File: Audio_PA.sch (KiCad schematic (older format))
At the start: 0 parts

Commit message: Electric circuit Ver_1
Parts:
- added C? (x2): 1uF, symbol C
- added C?: 330pF, symbol C
- added C?: 47uF, symbol CP1
- added C?: 10nF, symbol C
- added C? (x3): 100nF, symbol C
- added C?: 100uF, symbol CP1
- added C? (x2): 18pF, symbol C
- added C? (x2): 1000uF, symbol CP1
- added D? (x2): 15V, symbol D_Zener
- added D? (x2): 1N4148, symbol D
- added F? (x2): 3A, symbol Fuse
- added P?: Audio_In, symbol CONN_01X02
- added P?: -45VDC, symbol CONN_01X01
- added P?: Audio_Out, symbol CONN_01X02
- added P?: +45VDC, symbol CONN_01X01
- added Q? (x4): BCM856DS, symbol BCM856DS
- added Q? (x3): MJE350, symbol MJE350
- added Q? (x3): MJE340, symbol MJE340
- added Q?: BD139, symbol BD139
- added Q?: 2N3904, symbol Q_NPN_EBC
- added Q?: 2N3906, symbol Q_PNP_EBC
- added Q?: Q_NMOS_GDS, symbol Q_NMOS_GDS
- added Q?: Q_PMOS_GDS, symbol Q_PMOS_GDS
- added R?: 47K, symbol R
- added R?: 2K2, symbol R
- added R? (x3): 1K, symbol R
- added R? (x3): 470R, symbol R
- added R? (x4): 10K, symbol R
- added R? (x3): 100R, symbol R
- added R?: 27K, symbol R
- added R? (x2): 3K9, symbol R
- added R?: 10R, symbol R
- added R? (x4): R, symbol R
- added R? (x2): 0R33, symbol R
- added R? (x2): 330R, symbol R
- added RV?: 100R, symbol POT_TRIM
- added RV?: 1K, symbol POT_TRIM
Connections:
- new net: C?.1, C?.1, P?.1 (P1)
- new net: C?.2, C?.2, R?.1, R?.2
- new net: C?.1, Q?.2 (B), R?.1
- new net: Q?.1 (E), RV?.1
- new net: C?.2, Q?.3 (B), Q?.6 (C), R?.1
- new net: C?.1, Q?.3 (B), Q?.3 (C), R?.1
- new net: Q?.4 (E), RV?.3
- new net: Q?.5 (B), R?.1, R?.2
- new net: Q?.3 (C), RV?.2
- new net: C?.1, Q?.1 (E), Q?.1 (E), R?.1, R?.1, R?.1
- new net: Q?.2 (B), R?.1
- new net: Q?.5 (B), Q?.6 (C), R?.1
- new net: Q?.4 (E), R?.2, R?.2
- new net: C?.2, R?.1, R?.2
- new net: Q?.1 (E), R?.2 (x2)
- new net: Q?.2 (C), Q?.3 (B), Q?.3 (B), R?.1
- new net: C?.1, D?.1 (K), Q?.2 (C), Q?.2 (C), R?.1, R?.1
- new net: Q?.1 (E), Q?.1 (E), R?.1
- new net: C?.2, Q?.2 (C), R?.2
- new net: C?.1, C?.2, D?.2 (A), Q?.1 (E), Q?.2 (C), R?.1, R?.2
- new net: C?.1, C?.1, C?.1, R?.2
- new net: C?.1, D?.1 (K), D?.2 (A), P?.1 (P1), Q?.1 (E), Q?.1 (E), R?.1, R?.1, R?.1, R?.2, R?.2
- new net: Q?.1 (E), R?.2, R?.2, R?.2
- new net: F?.1, P?.1 (P1) (x2)
- new net: F?.2, Q?.2 (C), Q?.3 (S), R?.1
- new net: C?.2, R?.1
- new net: Q?.3 (B), R?.2, RV?.3
- new net: R?.1, RV?.1, RV?.2
- new net: D?.2 (A), Q?.1 (G), R?.2
- new net: D?.1 (K), Q?.1 (G), R?.2
- new net: D?.1 (K), Q?.3 (C)
- new net: D?.2 (A), Q?.3 (C)
- new net: Q?.2 (B), R?.1, R?.2 (x2)
- new net: Q?.3 (S), R?.1, R?.1
- new net: Q?.2 (D), R?.2, R?.2
- new net: F?.2, Q?.2 (C), Q?.2 (D), R?.1
- new net: C?.1, Q?.3 (B), R?.2
- new net: C?.2, Q?.3 (B), R?.2
- new net Earth: C?.1, C?.2, C?.2, C?.2, C?.2, P?.2 (P2), P?.2 (P2), R?.2, R?.2, R?.2

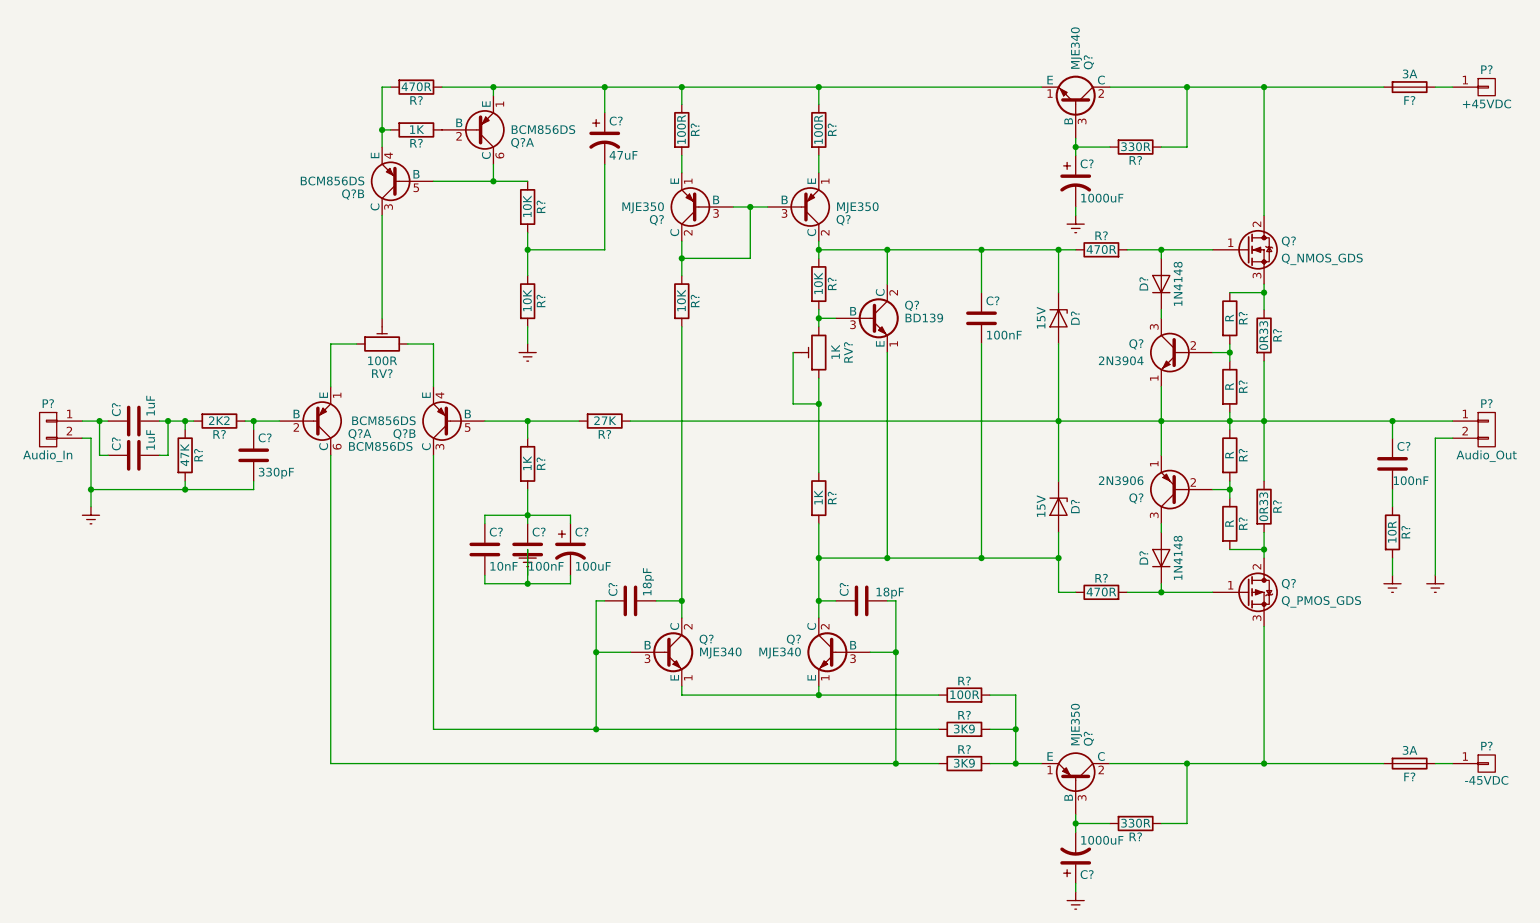
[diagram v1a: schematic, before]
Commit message: Electric circuit Ver_1.1
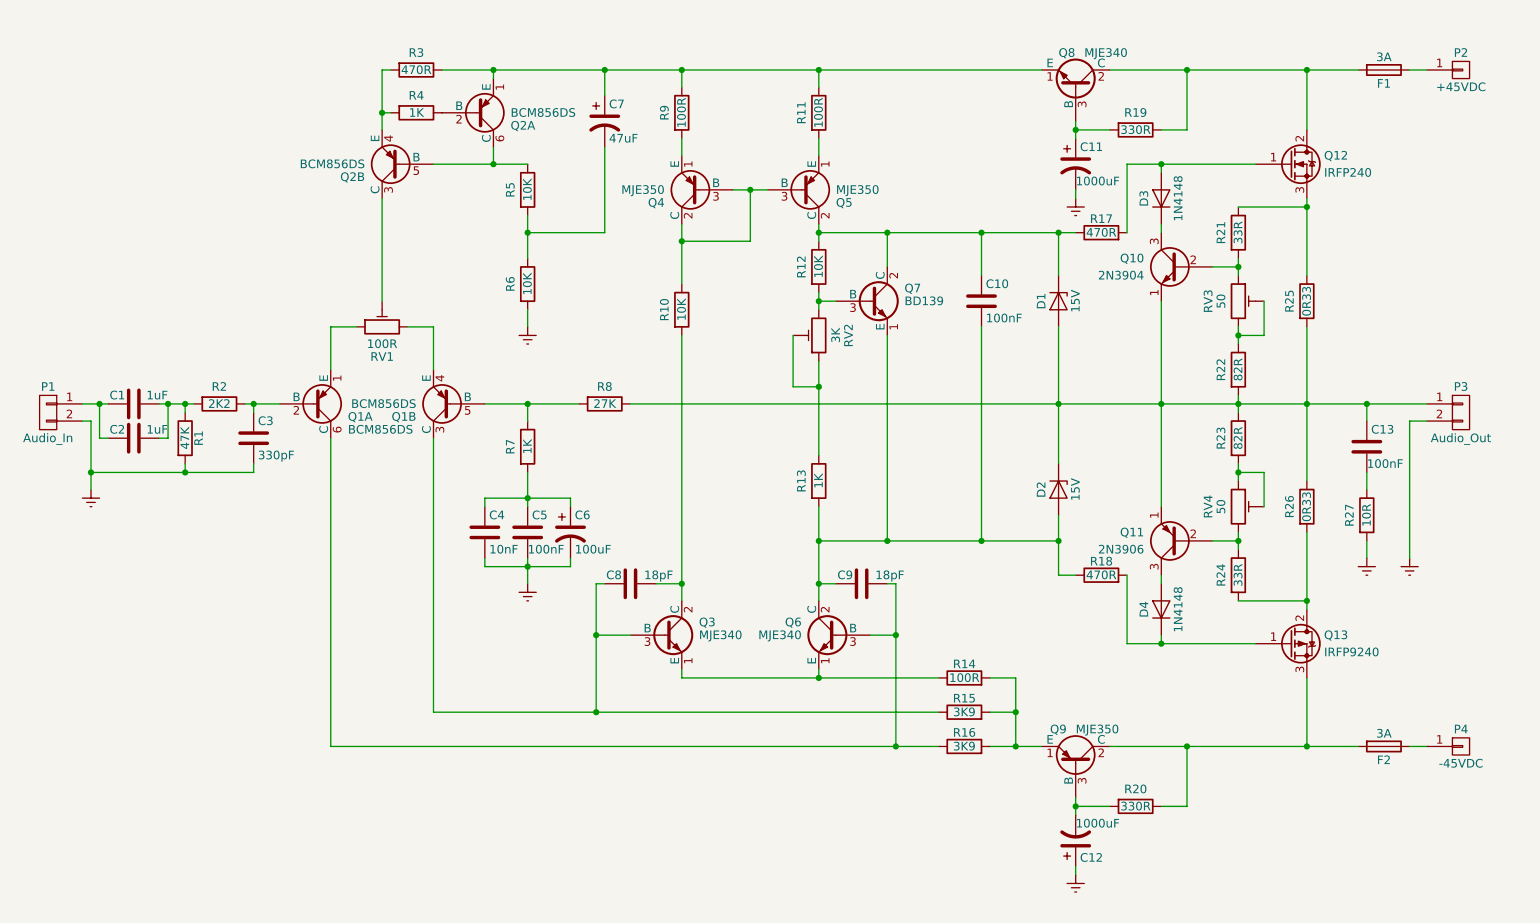
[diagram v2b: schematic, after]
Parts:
- removed R? (x2): R, symbol R
- added R23: 82R, symbol R
- added R24: 33R, symbol R
- added RV3, RV4: 50, symbol POT_TRIM
- Q12: renamed from Q?; value Q_NMOS_GDS -> IRFP240
- Q13: renamed from Q?; value Q_PMOS_GDS -> IRFP9240
- R21: renamed from R?; value R -> 33R
- R22: renamed from R?; value R -> 82R
- RV2: renamed from RV?; value 1K -> 3K
- gave numbers to parts that had none: 58
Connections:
- net Earth: now also C5.2
- net at C8.1, Q3.3 (B), R15.1: now also Q1.3 (C); no longer Q2.3 (C)
- net at RV1.3: now also Q1.4 (E); no longer Q2.4 (E)
- net at R7.1, R8.2: now also Q1.5 (B); no longer Q2.5 (B)
- net at RV1.2: now also Q2.3 (C); no longer Q1.3 (C)
- net at C7.1, Q8.1 (E), R11.1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: now also Q2.1 (E); no longer Q2.1 (E)
- net at R4.1: now also Q2.2 (B); no longer Q2.2 (B)
- net at R3.2, R4.2: now also Q2.4 (E); no longer Q1.4 (E)
- net at C13.1, D1.2 (A), D2.1 (K)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: now also R23.1
- net at Q10.2 (B), R21.2: now also RV3.1; no longer R22.1
- net at Q11.2 (B): now also R24.1, RV4.3
- net at Q13.2 (D), R26.2: now also R24.2
- new net: Q2.5 (B), Q2.6 (C), R5.1
- new net: R22.1, RV3.2, RV3.3
- new net: R23.2, RV4.1, RV4.2
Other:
- moved on the sheet: C1, C10, C11, C12, C13, C2, C3, C4, C5, C6, C7, C8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

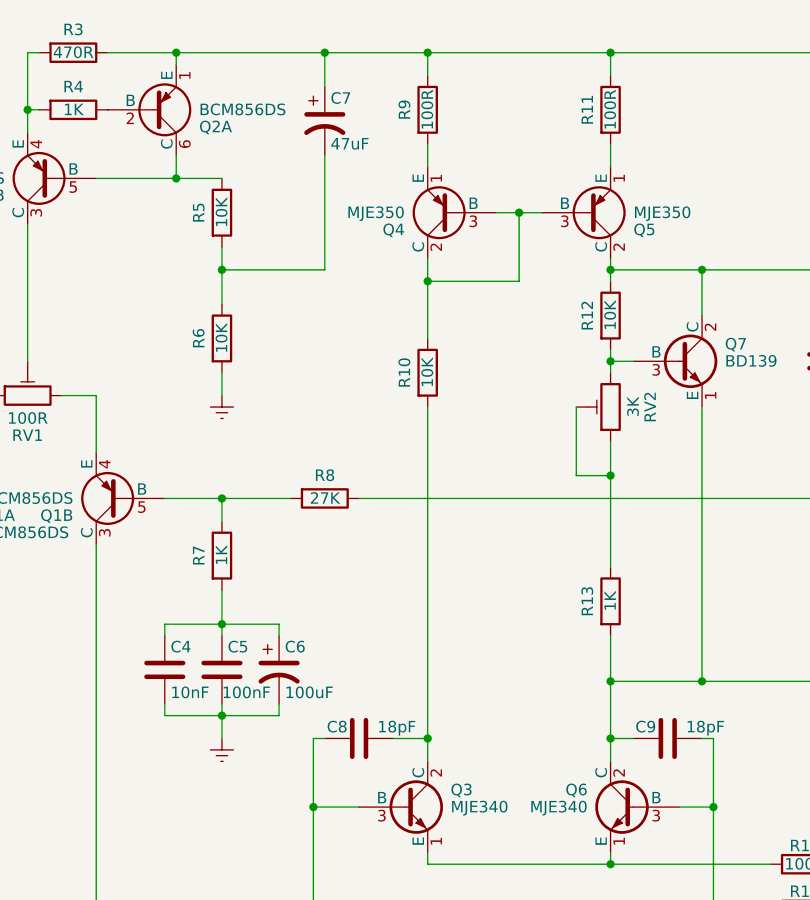
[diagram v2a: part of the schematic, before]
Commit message: Electric circuit Ver_1.2
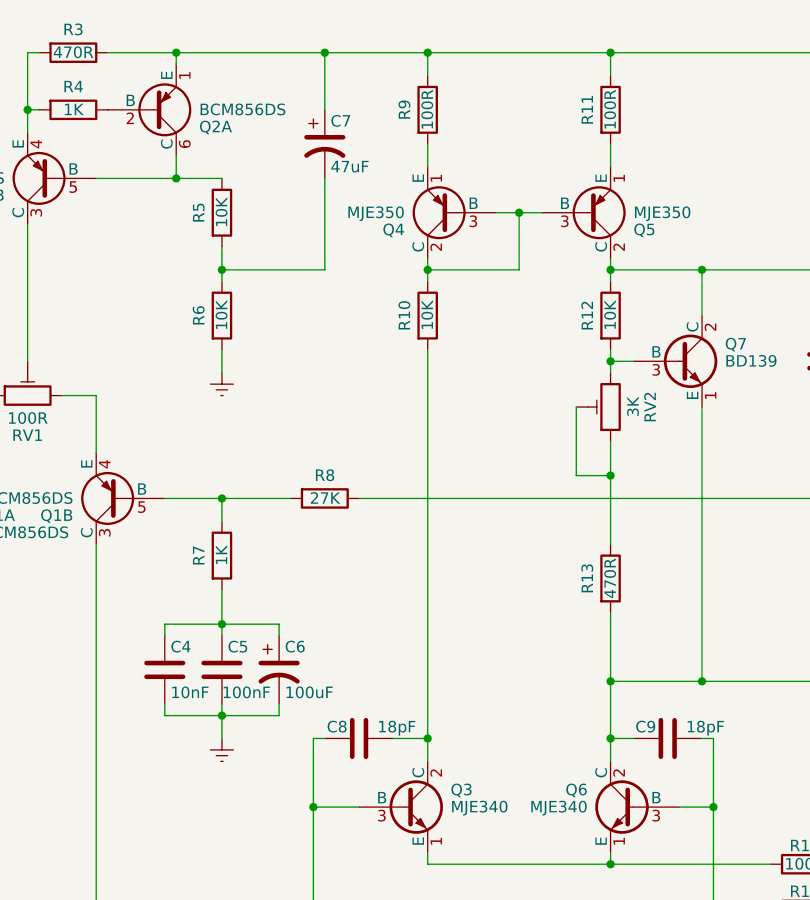
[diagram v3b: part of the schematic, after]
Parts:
- R13: value 1K -> 470R
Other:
- moved on the sheet: C7, R10, R13, R6
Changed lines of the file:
@@
 L R R6
 U 1 1 5872933E
-P 3950 2750
-F 0 "R6" V 3850 2750 50  0000 C CNN
-F 1 "10K" V 3950 2750 50  0000 C CNN
-F 2 "" V 3880 2750 50  0000 C CNN
-F 3 "" H 3950 2750 50  0000 C CNN
-	1    3950 2750
+P 3950 2650
+F 0 "R6" V 3850 2650 50  0000 C CNN
+F 1 "10K" V 3950 2650 50  0000 C CNN
+F 2 "" V 3880 2650 50  0000 C CNN
+F 3 "" H 3950 2650 50  0000 C CNN
+	1    3950 2650
 	1    0    0    -1
 $EndComp
@@
 L Earth #PWR2
 U 1 1 587293F8
-P 3950 3000
-F 0 "#PWR2" H 3950 2750 50  0001 C CNN
-F 1 "Earth" H 3950 2850 50  0001 C CNN
-F 2 "" H 3950 3000 50  0000 C CNN
-F 3 "" H 3950 3000 50  0000 C CNN
-	1    3950 3000
+P 3950 2900
+F 0 "#PWR2" H 3950 2650 50  0001 C CNN
+F 1 "Earth" H 3950 2750 50  0001 C CNN
+F 2 "" H 3950 2900 50  0000 C CNN
+F 3 "" H 3950 2900 50  0000 C CNN
+	1    3950 2900
 	1    0    0    -1
 $EndComp
@@
 L CP1 C7
 U 1 1 58729487
-P 4400 1800
-F 0 "C7" H 4425 1900 50  0000 L CNN
-F 1 "47uF" H 4425 1700 50  0000 L CNN
-F 2 "" H 4400 1800 50  0000 C CNN
-F 3 "" H 4400 1800 50  0000 C CNN
-	1    4400 1800
+P 4400 1900
+F 0 "C7" H 4425 2000 50  0000 L CNN
+F 1 "47uF" H 4425 1800 50  0000 L CNN
+F 2 "" H 4400 1900 50  0000 C CNN
+F 3 "" H 4400 1900 50  0000 C CNN
+	1    4400 1900
 	1    0    0    -1
 $EndComp
@@
 L R R10
 U 1 1 5872B168
-P 4850 2900
-F 0 "R10" V 4750 2900 50  0000 C CNN
-F 1 "10K" V 4850 2900 50  0000 C CNN
-F 2 "" V 4780 2900 50  0000 C CNN
-F 3 "" H 4850 2900 50  0000 C CNN
-	1    4850 2900
+P 4850 2650
+F 0 "R10" V 4750 2650 50  0000 C CNN
+F 1 "10K" V 4850 2650 50  0000 C CNN
+F 2 "" V 4780 2650 50  0000 C CNN
+F 3 "" H 4850 2650 50  0000 C CNN
+	1    4850 2650
 	1    0    0    -1
 $EndComp
@@
 L R R13
 U 1 1 58733360
-P 5650 3900
-F 0 "R13" V 5550 3900 50  0000 C CNN
-F 1 "1K" V 5650 3900 50  0000 C CNN
-F 2 "" V 5580 3900 50  0000 C CNN
-F 3 "" H 5650 3900 50  0000 C CNN
-	1    5650 3900
+P 5650 3800
+F 0 "R13" V 5550 3800 50  0000 C CNN
+F 1 "470R" V 5650 3800 50  0000 C CNN
+F 2 "" V 5580 3800 50  0000 C CNN
+F 3 "" H 5650 3800 50  0000 C CNN
+	1    5650 3800
 	1    0    0    -1
 $EndComp
@@
 	3950 2350 3950 2450
 Wire Wire Line
-	3950 2450 3950 2600
-Wire Wire Line
-	4400 1500 4400 1650
+	3950 2450 3950 2500
+Wire Wire Line
+	4400 1500 4400 1750
 Connection ~ 3750 1500
 Wire Wire Line
-	4400 1950 4400 2450
+	4400 2050 4400 2450
 Wire Wire Line
 	4400 2450 3950 2450
@@
 	5250 2200 5350 2200
 Wire Wire Line
-	5250 2200 5250 2500
-Wire Wire Line
-	5250 2500 4850 2500
-Wire Wire Line
-	4850 2400 4850 2500
-Wire Wire Line
-	4850 2500 4850 2750
+	5250 2200 5250 2450
+Wire Wire Line
+	5250 2450 4850 2450
+Wire Wire Line
+	4850 2400 4850 2450
+Wire Wire Line
+	4850 2450 4850 2500
 Connection ~ 5250 2200
 Wire Wire Line
@@
 Wire Wire Line
 	3700 4050 3700 4000
-Connection ~ 4850 2500
-Wire Wire Line
-	4850 3050 4850 4500
+Connection ~ 4850 2450
+Wire Wire Line
+	4850 2800 4850 4500
 Wire Wire Line
 	4850 4500 4850 4600
@@
 Connection ~ 5650 4500
 Wire Wire Line
-	3950 2900 3950 3000
+	3950 2800 3950 2900
 Connection ~ 5650 1500
 Wire Wire Line
@@
 	5650 2850 5650 2900
 Wire Wire Line
-	5650 4050 5650 4250
+	5650 3950 5650 4250
 Wire Wire Line
 	5650 4250 5650 4500
@@
 	5650 3200 5650 3350
 Wire Wire Line
-	5650 3350 5650 3750
+	5650 3350 5650 3650
 Wire Wire Line
 	5500 3050 5500 3350
